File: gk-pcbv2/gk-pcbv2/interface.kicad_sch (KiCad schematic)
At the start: 69 parts, among them J11 Conn_01x02, J7 Conn_01x02, Q1 MMBT3904, Q2 MMBT3904, SW3 RotaryEncoder_Switch, SW4 SW_DIP_x01, U9 LSM6DSL

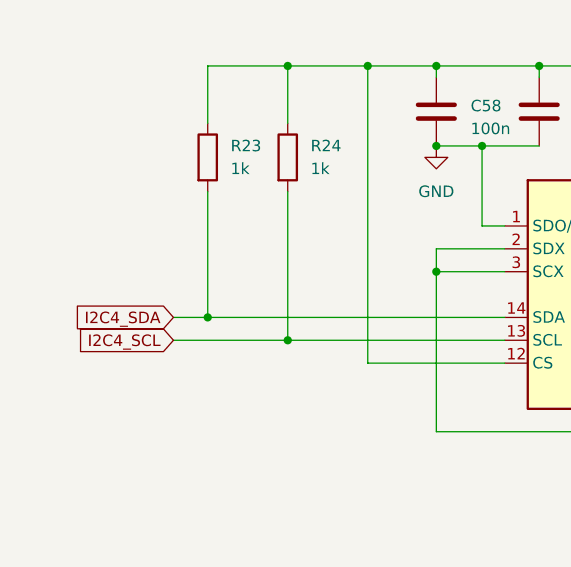
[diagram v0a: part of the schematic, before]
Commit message: more pcb changes
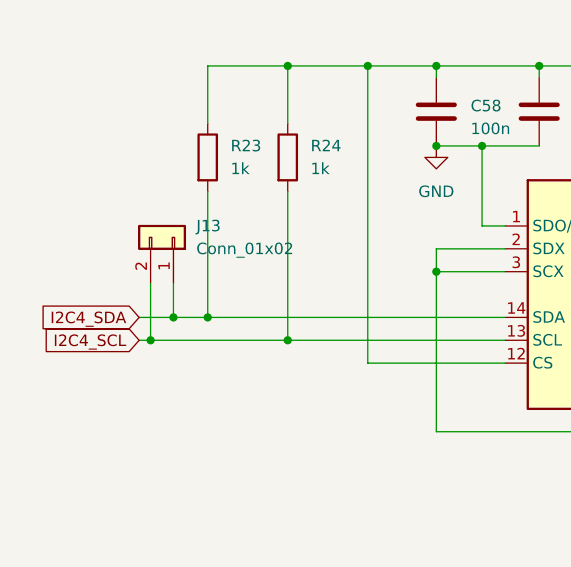
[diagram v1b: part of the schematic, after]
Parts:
- added J13: Conn_01x02, Connector_PinHeader_2.54mm:PinHeader_1x02_P2.54mm_Vertical, symbol Connector_Generic:Conn_01x02
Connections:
- net I2C4_SCL: now also J13.2 (Pin_2)
- net I2C4_SDA: now also J13.1 (Pin_1)
